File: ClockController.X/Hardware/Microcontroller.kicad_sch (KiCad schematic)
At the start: 3 parts, among them U1 PIC16F15224-I/SL

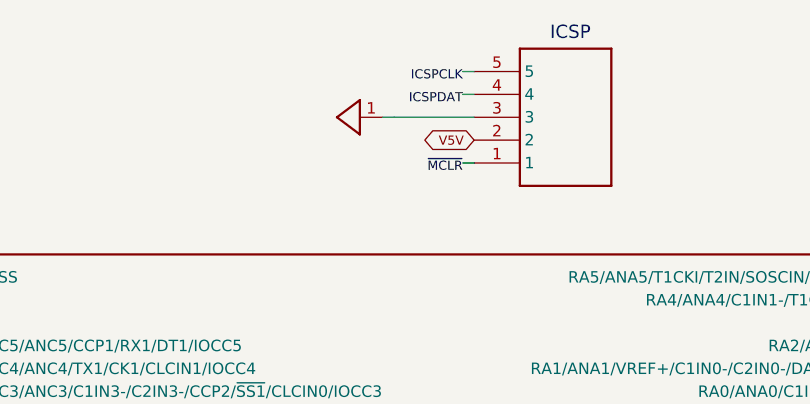
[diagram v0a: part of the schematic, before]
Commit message: Updated most footprints
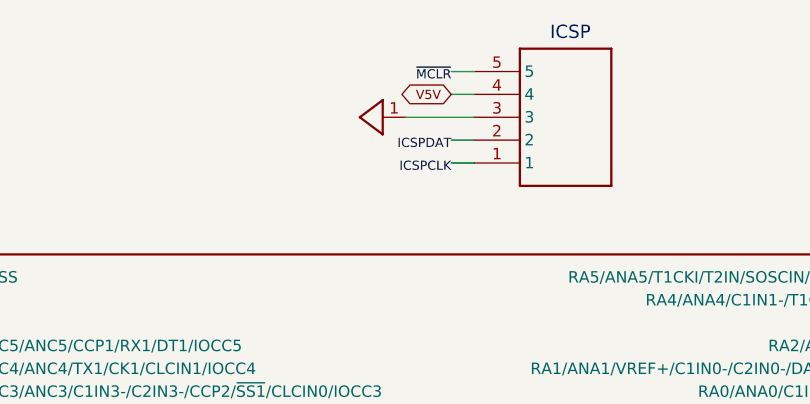
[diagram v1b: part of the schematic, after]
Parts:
- C2: footprint Clock Controller:CAP_0805 -> Capacitor_SMD:C_0805_2012Metric
- ICSP0: footprint Clock Controller:RHDRRA5W60P0X254_1X5_1320X850X274P -> Connector_PinSocket_2.54mm:PinSocket_1x05_P2.54mm_Horizontal
- U1: footprint Clock Controller:SOIC14P127_869X599X175L84X42N -> Package_SO:SOIC-14_3.9x8.7mm_P1.27mm
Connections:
- net ICSPCLK: now also ICSP0.1; no longer ICSP0.5
- net ICSPDAT: now also ICSP0.2; no longer ICSP0.4
- net V5V: now also ICSP0.4; no longer ICSP0.2
- net ~{MCLR}: now also ICSP0.5; no longer ICSP0.1
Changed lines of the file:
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@@
+	(wire
+		(pts
+			(xy 135.89 77.47) (xy 138.43 77.47)
+		)
+		(stroke
+			(width 0)
+			(type default)
+		)
+	)
 	(wire
 		(pts
@@
 	(wire
 		(pts
-			(xy 129.54 82.55) (xy 128.27 82.55)
-		)
-		(stroke
-			(width 0.25)
-			(type solid)
-		)
-	)
-	(wire
-		(pts
 			(xy 78.74 107.95) (xy 80.01 107.95)
 		)
@@
 	(wire
 		(pts
+			(xy 135.89 80.01) (xy 138.43 80.01)
+		)
+		(stroke
+			(width 0)
+			(type default)
+		)
+	)
+	(wire
+		(pts
 			(xy 209.55 102.87) (xy 207.01 102.87)
 		)
@@
 	(wire
 		(pts
-			(xy 138.43 87.63) (xy 137.16 87.63)
-		)
-		(stroke
-			(width 0)
-			(type default)
-		)
-	)
-	(wire
-		(pts
 			(xy 78.74 118.11) (xy 80.01 118.11)
 		)
@@
 	(wire
 		(pts
+			(xy 135.89 87.63) (xy 138.43 87.63)
+		)
+		(stroke
+			(width 0)
+			(type default)
+		)
+	)
+	(wire
+		(pts
+			(xy 130.81 82.55) (xy 138.43 82.55)
+		)
+		(stroke
+			(width 0)
+			(type default)
+		)
+	)
+	(wire
+		(pts
 			(xy 205.74 130.81) (xy 147.32 130.81)
 		)
@@
 	(wire
 		(pts
-			(xy 137.16 80.01) (xy 138.43 80.01)
-		)
-		(stroke
-			(width 0)
-			(type default)
-		)
-	)
-	(wire
-		(pts
 			(xy 78.74 120.65) (xy 80.01 120.65)
 		)
@@
 	(wire
 		(pts
-			(xy 137.16 77.47) (xy 138.43 77.47)
-		)
-		(stroke
-			(width 0)
-			(type default)
-		)
-	)
-	(wire
-		(pts
-			(xy 129.54 82.55) (xy 138.43 82.55)
-		)
-		(stroke
-			(width 0)
-			(type default)
-		)
-	)
-	(wire
-		(pts
 			(xy 209.55 102.87) (xy 205.74 102.87)
 		)
@@
 			(width 0.25)
 			(type solid)
+		)
+	)
+	(wire
+		(pts
+			(xy 135.89 85.09) (xy 138.43 85.09)
+		)
+		(stroke
+			(width 0)
+			(type default)
 		)
 	)
@@
 	)
 	(label "ICSPDAT"
-		(at 137.16 80.01 180)
+		(at 135.89 85.09 180)
 		(fields_autoplaced yes)
 		(effects
@@
 	)
 	(label "~{MCLR}"
-		(at 137.16 87.63 180)
+		(at 135.89 77.47 180)
 		(fields_autoplaced yes)
 		(effects
@@
 	)
 	(label "ICSPCLK"
-		(at 137.16 77.47 180)
+		(at 135.89 87.63 180)
 		(fields_autoplaced yes)
 		(effects
@@
 	(global_label "V5V"
 		(shape bidirectional)
-		(at 138.43 85.09 180)
+		(at 135.89 80.01 180)
 		(fields_autoplaced yes)
 		(effects
@@
 		)
 		(property "Intersheetrefs" "${INTERSHEET_REFS}"
-			(at 132.4437 85.09 0)
+			(at 129.9037 80.01 0)
 			(effects
 				(font
@@
 			)
 		)
-		(property "Footprint" "Clock Controller:SOIC14P127_869X599X175L84X42N"
+		(property "Footprint" "Package_SO:SOIC-14_3.9x8.7mm_P1.27mm"
 			(at 143.51 110.49 0)
 			(effects
@@
 	(symbol
 		(lib_id "Clock Controller-eagle-import:GND_DIGITAL")
-		(at 124.46 82.55 270)
+		(at 127 82.55 270)
 		(unit 1)
 		(exclude_from_sim no)
@@
 		(dnp no)
 		(property "Reference" "#NetPort04"
-			(at 124.46 82.55 0)
+			(at 127 82.55 0)
 			(effects
 				(font
@@
 		)
 		(property "Value" "GND_DIGITAL"
-			(at 124.46 82.55 0)
+			(at 127 82.55 0)
 			(effects
 				(font
@@
 		)
 		(property "Footprint" ""
-			(at 124.46 82.55 0)
+			(at 127 82.55 0)
 			(effects
 				(font
@@
 		)
 		(property "Datasheet" ""
-			(at 124.46 82.55 0)
+			(at 127 82.55 0)
 			(effects
 				(font
@@
 		)
 		(property "Description" ""
-			(at 124.46 82.55 0)
+			(at 127 82.55 0)
 			(effects
 				(font
@@
 			)
 		)
-		(property "Footprint" "Clock Controller:RHDRRA5W60P0X254_1X5_1320X850X274P"
+		(property "Footprint" "Connector_PinSocket_2.54mm:PinSocket_1x05_P2.54mm_Horizontal"
 			(at 138.43 87.63 0)
 			(effects
@@
 			)
 		)
-		(property "Footprint" "Clock Controller:CAP_0805"
+		(property "Footprint" "Capacitor_SMD:C_0805_2012Metric"
 			(at 143.51 130.81 0)
 			(effects
